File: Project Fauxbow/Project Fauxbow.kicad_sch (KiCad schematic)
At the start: 41 parts, among them K10 Kailh Hotswap Socket, K11 Kailh Hotswap Socket, K12 Kailh Hotswap Socket, K13 Kailh Hotswap Socket, K14 Kailh Hotswap Socket, K15 Kailh Hotswap Socket, K16 Kailh Hotswap Socket, K2 Kailh Hotswap Socket, K3 Kailh Hotswap Socket, K4 Kailh Hotswap Socket, K5 Kailh Hotswap Socket, K6 Kailh Hotswap Socket, K7 Kailh Hotswap Socket, K8 Kailh Hotswap Socket, K9 Kailh Hotswap Socket

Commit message: current
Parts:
- removed D1, D10, D11, D12, D13, D14, D15, D16, D2, D3, D4, D5, D6, D7, D8, D9: 1N4148, Diode_SMD:D_SOD-123, symbol Device:D_Small
- removed U2: (no value), symbol Regulator_Linear:AP2112K-3.3
- added C3, C4: 10u, Capacitor_SMD:C_0805_2012Metric, symbol Device:C_Small
- added D22, D23, D24, D25, D26, D27, D28, D29, D30, D31, D32, D33, D34, D35, D36, D37, D38, D39, D40: SK6812MINI, marbastlib-mx:LED_MX_6028R-FLIPPED, symbol LED:SK6812MINI
- added H1, H2, H3, H4, H5, H6: MountingHole_Pad, MountingHole:MountingHole_2.7mm_M2.5_ISO7380_Pad, symbol Mechanical:MountingHole_Pad
- added J2: USB 1, Connector_USB:USB_A_Stewart_SS-52100-001_Horizontal, symbol Connector:USB_A
- added J3: USB 2, Connector_USB:USB_A_Stewart_SS-52100-001_Horizontal, symbol Connector:USB_A
- added J4: USB 3, Connector_USB:USB_A_Stewart_SS-52100-001_Horizontal, symbol Connector:USB_A
- added K10, K15, K20, K5: Kailh Hotswap Socket, marbastlib-mx:SW_MX_HS_1u, symbol Switch:SW_Push
- added R3, R4: 5.1k, Resistor_SMD:R_0805_2012Metric, symbol Device:R_Small
- added R5: 2.7k, Resistor_SMD:R_0805_2012Metric, symbol Device:R_Small
- added U2: AP1117-33, Package_TO_SOT_SMD:SOT-223-3_TabPin2, symbol Regulator_Linear:AP1117-33
- added U3: FE1.1, Package_QFP:LQFP-48_7x7mm_P0.5mm, symbol index:FE1.1
- added Y2: 12MHz, Crystal:Crystal_SMD_3225-4Pin_3.2x2.5mm, symbol Device:Crystal_GND24_Small
- C1, C2: value (none) -> 22pF; footprint (none) -> Capacitor_SMD:C_1206_3216Metric_Pad1.33x1.80mm_HandSolder
- D21: renamed from D17; value (none) -> SK6812MINI; footprint (none) -> marbastlib-mx:LED_MX_6028R-FLIPPED
- J1: value (none) -> Host; footprint (none) -> Connector_USB:USB_C_Receptacle_Palconn_UTC16-G; Digikey (none) -> 2073-USB4105-GF-ACT-ND; JLCPCB (none) -> C165948; LCSC (none) -> C165948
- K1: value (none) -> Kailh Hotswap Socket; footprint (none) -> marbastlib-mx:SW_MX_HS_1u
- R1: value (none) -> 10k; footprint (none) -> Resistor_SMD:R_1206_3216Metric_Pad1.30x1.75mm_HandSolder
- SW1: value (none) -> SW_Push; footprint (none) -> keebs:SW_Tactile_SPST_Angled_MJTP1117
- U1: value (none) -> ATmega32U4-A; footprint (none) -> Package_QFP:TQFP-44_10x10mm_P0.8mm
- Y1: value (none) -> 16MHz; footprint (none) -> Oscillator:Oscillator_SMD_Abracon_ASE-4Pin_3.2x2.5mm_HandSoldering
- renumbered K9 to K11, K10 to K12, K11 to K13, K12 to K14, K13 to K16, K14 to K17, K15 to K18, K16 to K19, K5 to K6, K6 to K7, K7 to K8, K8 to K9
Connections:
- net USB GND is gone; now on net GND: U1.5 (UGND)
- net VCC is gone; now on net VBUS: R1.1, U1.14 (VCC), U1.24 (AVCC), U1.34 (VCC), U1.44 (AVCC)
- net row2 is gone; now on net key_6: U1.29 (PB5)
- net row3 is gone; now on net key_7: U1.30 (PB6)
- net row4 is gone; now on net key_8: U1.12 (PB7)
- net GND: now also D21.2 (VSS), J1.S1 (SHIELD), K1.1, K11.1, K12.1, K13.1, K14.1, K16.1, K17.1, K18.1, K19.1, K2.1, K3.1, K4.1, K6.1, K7.1, K8.1, K9.1, C3.2, C4.2, D22.2 (VSS), D23.2 (VSS), D24.2 (VSS), D25.2 (VSS), D26.2 (VSS), D27.2 (VSS), D28.2 (VSS), D29.2 (VSS), D30.2 (VSS), D31.2 (VSS), D32.2 (VSS), D33.2 (VSS), D34.2 (VSS), D35.2 (VSS), D36.2 (VSS), D37.2 (VSS), D38.2 (VSS), D39.2 (VSS), D40.2 (VSS), J2.4 (GND), J2.5 (Shield), J3.4 (GND), J3.5 (Shield), J4.4 (GND), J4.5 (Shield), K10.1, K15.1, K20.1, K5.1, R3.2, R4.2, R5.2, U2.1 (GND), U3.1 (OVCB2), U3.10 (VS_PLL), U3.16 (VSS), U3.22 (VSS), U3.25 (VS_A), U3.33 (VSS), U3.40 (TEST), U3.46 (LED4), U3.5 (OVCB3), U3.6 (VSS), U3.7 (OVCB4), U3.8 (PWRB4), Y2.2, Y2.4
- net key_7: now reaches K7.2
- net key_9: now reaches K9.2
- net key_9: now also U1.31 (PC6)
- net key_12: now reaches K12.2
- net key_12: now also U1.19 (PD1)
- net key_18: now reaches K18.2
- net key_18: now also U1.27 (PD7)
- net key_16: now reaches K16.2
- net key_16: now also U1.22 (PD5)
- net key_19: now reaches K19.2
- net key_19: now also U1.41 (PF0)
- net key_13: now reaches K13.2
- net key_13: now also U1.20 (PD2)
- net key_17: now reaches K17.2
- net key_17: now also U1.26 (PD6)
- net key_3: now reaches K3.2
- net key_3: now also U1.10 (PB2)
- net key_8: now reaches K8.2
- net key_6: now reaches K6.2
- net key_1: now reaches K1.2
- net key_1: now also U1.8 (PB0)
- net key_11: now reaches K11.2
- net key_11: now also U1.18 (PD0)
- net key_14: now reaches U1.21 (PD3)
- net key_14: now also K14.2
- net key_15: now reaches U1.25 (PD4)
- net key_15: now also K15.2
- net key_10: now reaches U1.32 (PC7)
- net key_10: now also K10.2
- net LED: now reaches U1.36 (PF7)
- net LED: now also D21.3 (DIN)
- net key_20: now reaches U1.40 (PF1)
- net key_20: now also K20.2
- net VBUS: now reaches U1.7 (VBUS)
- net VBUS: now also D21.4 (VDD), J1.A4 (VBUS), J1.A9 (VBUS), J1.B4 (VBUS), J1.B9 (VBUS), D22.4 (VDD), D23.4 (VDD), D24.4 (VDD), D25.4 (VDD), D26.4 (VDD), D27.4 (VDD), D28.4 (VDD), D29.4 (VDD), D30.4 (VDD), D31.4 (VDD), D32.4 (VDD), D33.4 (VDD), D34.4 (VDD), D35.4 (VDD), D36.4 (VDD), D37.4 (VDD), D38.4 (VDD), D39.4 (VDD), D40.4 (VDD), J2.1 (VBUS), J3.1 (VBUS), J4.1 (VBUS), U2.3 (VI), U3.35 (VBUSM)
- net key_4: now reaches K4.2
- net key_4: now also U1.11 (PB3)
- net key_2: now reaches K2.2
- net key_2: now also U1.9 (PB1)
- net at D21.1 (DOUT): now also D26.3 (DIN)
- net +BATT: no longer names the net of U1.2 (UVCC)
- net CC1: no longer names the net of J1.A5 (CC1)
- net CC1: now also R4.1
- net CC2: no longer names the net of J1.B5 (CC2)
- net CC2: now also R3.1
- net D+ renamed MD+
- net MD+: now also U3.31 (DPU); no longer U1.4 (D+)
- net D- renamed MD-
- net MD-: now also U3.30 (DMU); no longer U1.3 (D-)
- removed net col1: K1.1, K2.1, K3.1, K4.1, U1.8 (PB0)
- removed net col2: K6.1, K7.1, K8.1, K9.1, U1.9 (PB1)
- removed net col3: K11.1, K12.1, K13.1, K14.1, U1.10 (PB2)
- removed net col4: K16.1, K17.1, K18.1, K19.1, U1.11 (PB3)
- net row1 renamed key_5
- net key_5: now also K5.2
- new net: D24.3 (DIN), D29.1 (DOUT)
- new net: D29.3 (DIN), D34.1 (DOUT)
- new net: D28.1 (DOUT), D33.3 (DIN)
- new net: D23.1 (DOUT), D28.3 (DIN)
- new net: D36.1 (DOUT), D37.3 (DIN)
- new net: D31.1 (DOUT), D36.3 (DIN)
- new net: D35.1 (DOUT), D40.3 (DIN)
- new net: D30.1 (DOUT), D35.3 (DIN)
- new net: D27.3 (DIN), D32.1 (DOUT)
- new net: D32.3 (DIN), D37.1 (DOUT)
- new net: D26.1 (DOUT), D31.3 (DIN)
- new net: D22.1 (DOUT), D23.3 (DIN)
- new net: D34.3 (DIN), D39.1 (DOUT)
- new net: D38.1 (DOUT), D39.3 (DIN)
- new net: D25.1 (DOUT), D30.3 (DIN)
- new net: D33.1 (DOUT), D38.3 (DIN)
- new net: D22.3 (DIN), D27.1 (DOUT)
- new net: R5.1, U3.28 (REXT)
- new net: D24.1 (DOUT), D25.3 (DIN)
- new net: U3.11 (XOUT), Y2.1
- new net: U3.12 (XIN), Y2.3
- new net +3V3: C3.1, U2.2 (VO), U3.13 (VD33), U3.19 (VD33), U3.27 (VD3_IN), U3.32 (VD33), U3.34 (~{XRSTJ}), U3.36 (BUS_B), U3.37 (DIS_REG), U3.41 (VD33), U3.48 (OVCB1)
- new net 1.8: C4.1, U3.26 (VREG18), U3.29 (VD18), U3.3 (VD18), U3.9 (VD_PLL)
- new net 1D+: J2.3 (D+), U3.24 (DP1)
- new net 1D-: J2.2 (D-), U3.23 (DM1)
- new net 2D+: J3.3 (D+), U3.21 (DP2)
- new net 2D-: J3.2 (D-), U3.20 (DM2)
- new net 3D+: J4.3 (D+), U3.18 (DP3)
- new net 3D-: J4.2 (D-), U3.17 (DM3)
- new net 4D+: U1.4 (D+), U3.15 (DP4)
- new net 4D-: U1.3 (D-), U3.14 (DM4)
- new net DRV: U3.42 (DRV)
- no-connect marks 0 -> 10
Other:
- note added: "32u4 BB"
- note added: "3V3 linear regulator"
- note added: "Connection to PC"
- note added: "Hub"
- note added: "Keyswitch Array (mx kaihl hotswap 5 pin holey bois)"
- note added: "Lord Mountyboiks"
- note added: "Ports"
- note added: "RGB LED Array Gal"
- note added: "Reset Thembo"
- note removed: "Switch Array"
- moved on the sheet: C1, C2, D21, K1, K11, K12, K13, K14, K16, K17, K18, K19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

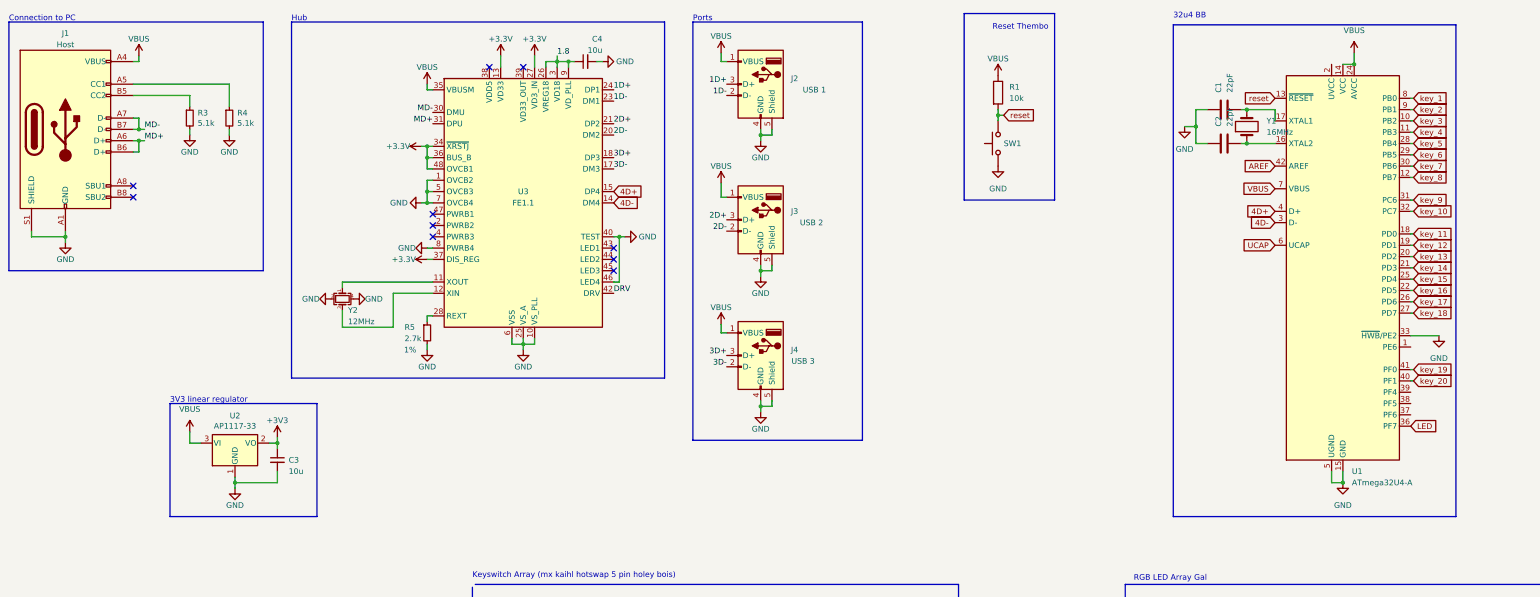
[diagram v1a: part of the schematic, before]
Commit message: INITIAL COMMIT REV 1
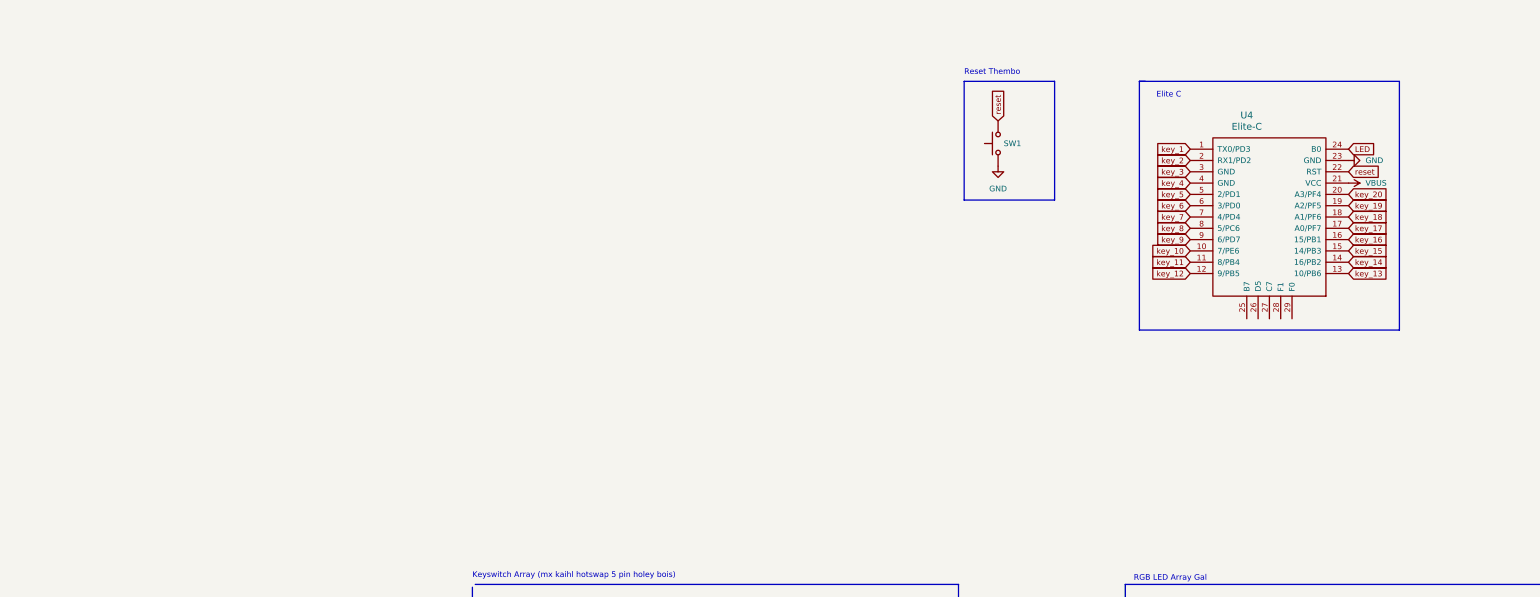
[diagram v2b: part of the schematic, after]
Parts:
- removed C1, C2: 22pF, Capacitor_SMD:C_1206_3216Metric_Pad1.33x1.80mm_HandSolder, symbol Device:C
- removed C3, C4: 10u, Capacitor_SMD:C_0805_2012Metric, symbol Device:C_Small
- removed J1: Host, Connector_USB:USB_C_Receptacle_Palconn_UTC16-G, symbol Connector:USB_C_Receptacle_USB2.0
- removed J2: USB 1, Connector_USB:USB_A_Stewart_SS-52100-001_Horizontal, symbol Connector:USB_A
- removed J3: USB 2, Connector_USB:USB_A_Stewart_SS-52100-001_Horizontal, symbol Connector:USB_A
- removed J4: USB 3, Connector_USB:USB_A_Stewart_SS-52100-001_Horizontal, symbol Connector:USB_A
- removed R1: 10k, Resistor_SMD:R_1206_3216Metric_Pad1.30x1.75mm_HandSolder, symbol Device:R
- removed R3, R4: 5.1k, Resistor_SMD:R_0805_2012Metric, symbol Device:R_Small
- removed R5: 2.7k, Resistor_SMD:R_0805_2012Metric, symbol Device:R_Small
- removed U1: ATmega32U4-A, Package_QFP:TQFP-44_10x10mm_P0.8mm, symbol MCU_Microchip_ATmega:ATmega32U4-A
- removed U2: AP1117-33, Package_TO_SOT_SMD:SOT-223-3_TabPin2, symbol Regulator_Linear:AP1117-33
- removed U3: FE1.1, Package_QFP:LQFP-48_7x7mm_P0.5mm, symbol index:FE1.1
- removed Y1: 16MHz, Oscillator:Oscillator_SMD_Abracon_ASE-4Pin_3.2x2.5mm_HandSoldering, symbol Device:Crystal
- removed Y2: 12MHz, Crystal:Crystal_SMD_3225-4Pin_3.2x2.5mm, symbol Device:Crystal_GND24_Small
- added U4: Elite-C, keebs:Elite-C-castellated-29pin-holes, symbol Keebs:Elite-C
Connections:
- net GND: now also U4.23 (GND)
- net LED: now also U4.24 (B0)
- net VBUS: now also U4.21 (VCC)
- net key_1: now also U4.1 (TX0/PD3)
- net key_10: now also U4.10 (7/PE6)
- net key_11: now also U4.11 (8/PB4)
- net key_12: now also U4.12 (9/PB5)
- net key_13: now also U4.13 (10/PB6)
- net key_14: now also U4.14 (16/PB2)
- net key_15: now also U4.15 (14/PB3)
- net key_16: now also U4.16 (15/PB1)
- net key_17: now also U4.17 (A0/PF7)
- net key_18: now also U4.18 (A1/PF6)
- net key_19: now also U4.19 (A2/PF5)
- net key_2: now also U4.2 (RX1/PD2)
- net key_20: now also U4.20 (A3/PF4)
- net key_3: now also U4.3 (GND)
- net key_4: now also U4.4 (GND)
- net key_5: now also U4.5 (2/PD1)
- net key_6: now also U4.6 (3/PD0)
- net key_7: now also U4.7 (4/PD4)
- net key_8: now also U4.8 (5/PC6)
- net key_9: now also U4.9 (6/PD7)
- net reset: now also U4.22 (RST)
- no-connect marks 10 -> 0
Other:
- note added: "Elite C"
- note removed: "32u4 BB"
- note removed: "3V3 linear regulator"
- note removed: "Connection to PC"
- note removed: "Hub"
- note removed: "Ports"
